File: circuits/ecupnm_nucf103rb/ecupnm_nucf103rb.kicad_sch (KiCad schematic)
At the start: 45 parts, among them J1 Conn_01x02_Pin, J2 Conn_01x02_Pin, J3 Conn_01x02_Pin, J4 Conn_01x03_Pin, J5 USB_B_Mini, U1 NUCLEO-64, U3 AMS1117-5.0

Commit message: Nucleo 64
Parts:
- C4: footprint (none) -> Capacitor_SMD:C_1206_3216Metric_Pad1.33x1.80mm_HandSolder
- C? (x4): footprint Capacitor_SMD:C_0805_2012Metric_Pad1.18x1.45mm_HandSolder -> Capacitor_SMD:C_1206_3216Metric_Pad1.33x1.80mm_HandSolder
- D3: footprint (none) -> LED_SMD:LED_1206_3216Metric_Pad1.42x1.75mm_HandSolder
- D?: footprint LED_SMD:LED_0805_2012Metric_Pad1.15x1.40mm_HandSolder -> LED_SMD:LED_1206_3216Metric_Pad1.42x1.75mm_HandSolder
- J1, J2, J3: footprint (none) -> Connector_PinSocket_2.54mm:PinSocket_1x02_P2.54mm_Vertical
- J4: footprint (none) -> Connector_PinSocket_2.54mm:PinSocket_1x03_P2.54mm_Vertical
- J5: footprint (none) -> Connector_USB:USB_Mini-B_Wuerth_65100516121_Horizontal
- JT1: footprint (none) -> TerminalBlock:TerminalBlock_Altech_AK300-3_P5.00mm
- JT2, JT3: footprint (none) -> TerminalBlock:TerminalBlock_Altech_AK300-2_P5.00mm
- R8, R9: footprint (none) -> Resistor_SMD:R_1206_3216Metric_Pad1.30x1.75mm_HandSolder
- R? (x13): footprint Resistor_SMD:R_0805_2012Metric_Pad1.20x1.40mm_HandSolder -> Resistor_SMD:R_1206_3216Metric_Pad1.30x1.75mm_HandSolder
- U1: footprint MODULE -> user:Nucleo-64
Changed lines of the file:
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@@
       (effects (font (size 1.27 1.27)))
     )
-    (property "Footprint" "" (at 139.7 51.1048 0)
+    (property "Footprint" "Capacitor_SMD:C_1206_3216Metric_Pad1.33x1.80mm_HandSolder" (at 139.7 51.1048 0)
       (effects (font (size 1.27 1.27)) hide)
     )
@@
       (effects (font (size 1.27 1.27)) hide)
     )
-    (property "Footprint" "" (at 114.3 119.38 0)
+    (property "Footprint" "Connector_PinSocket_2.54mm:PinSocket_1x02_P2.54mm_Vertical" (at 114.3 119.38 0)
       (effects (font (size 1.27 1.27)) hide)
     )
@@
       (effects (font (size 1.27 1.27)) (justify left))
     )
-    (property "Footprint" "Resistor_SMD:R_0805_2012Metric_Pad1.20x1.40mm_HandSolder" (at 94.742 104.14 90)
+    (property "Footprint" "Resistor_SMD:R_1206_3216Metric_Pad1.30x1.75mm_HandSolder" (at 94.742 104.14 90)
       (effects (font (size 1.27 1.27)) hide)
     )
@@
       (effects (font (size 1.27 1.27)) (justify left))
     )
-    (property "Footprint" "Resistor_SMD:R_0805_2012Metric_Pad1.20x1.40mm_HandSolder" (at 122.682 104.14 90)
+    (property "Footprint" "Resistor_SMD:R_1206_3216Metric_Pad1.30x1.75mm_HandSolder" (at 122.682 104.14 90)
       (effects (font (size 1.27 1.27)) hide)
     )
@@
       (effects (font (size 1.27 1.27)) (justify left))
     )
-    (property "Footprint" "Capacitor_SMD:C_0805_2012Metric_Pad1.18x1.45mm_HandSolder" (at 105.1052 175.26 0)
+    (property "Footprint" "Capacitor_SMD:C_1206_3216Metric_Pad1.33x1.80mm_HandSolder" (at 105.1052 175.26 0)
       (effects (font (size 1.27 1.27)) hide)
     )
@@
       (effects (font (size 1.27 1.27)) hide)
     )
-    (property "Footprint" "" (at 30.48 166.37 0)
+    (property "Footprint" "TerminalBlock:TerminalBlock_Altech_AK300-3_P5.00mm" (at 30.48 166.37 0)
       (effects (font (size 1.27 1.27)) hide)
     )
@@
       (effects (font (size 1.27 1.27)) (justify right))
     )
-    (property "Footprint" "LED_SMD:LED_0805_2012Metric_Pad1.15x1.40mm_HandSolder" (at 88.9 114.3 0)
+    (property "Footprint" "LED_SMD:LED_1206_3216Metric_Pad1.42x1.75mm_HandSolder" (at 88.9 114.3 0)
       (effects (font (size 1.27 1.27)) hide)
     )
@@
       (effects (font (size 1.27 1.27)))
     )
-    (property "Footprint" "Resistor_SMD:R_0805_2012Metric_Pad1.20x1.40mm_HandSolder" (at 166.37 47.498 90)
+    (property "Footprint" "Resistor_SMD:R_1206_3216Metric_Pad1.30x1.75mm_HandSolder" (at 166.37 47.498 90)
       (effects (font (size 1.27 1.27)) hide)
     )
@@
       (effects (font (size 1.27 1.27)) hide)
     )
-    (property "Footprint" "" (at 86.36 162.56 0)
+    (property "Footprint" "TerminalBlock:TerminalBlock_Altech_AK300-2_P5.00mm" (at 86.36 162.56 0)
       (effects (font (size 1.27 1.27)) hide)
     )
@@
       (effects (font (size 1.27 1.27)))
     )
-    (property "Footprint" "Resistor_SMD:R_0805_2012Metric_Pad1.20x1.40mm_HandSolder" (at 223.52 47.498 90)
+    (property "Footprint" "Resistor_SMD:R_1206_3216Metric_Pad1.30x1.75mm_HandSolder" (at 223.52 47.498 90)
       (effects (font (size 1.27 1.27)) hide)
     )
@@
       (effects (font (size 1.27 1.27)) (justify left))
     )
-    (property "Footprint" "Resistor_SMD:R_0805_2012Metric_Pad1.20x1.40mm_HandSolder" (at 74.422 120.65 90)
+    (property "Footprint" "Resistor_SMD:R_1206_3216Metric_Pad1.30x1.75mm_HandSolder" (at 74.422 120.65 90)
       (effects (font (size 1.27 1.27)) hide)
     )
@@
       (effects (font (size 1.27 1.27)))
     )
-    (property "Footprint" "MODULE" (at 113.03 22.86 0)
+    (property "Footprint" "user:Nucleo-64" (at 113.03 22.86 0)
       (effects (font (size 1.27 1.27)) hide)
     )
@@
       (effects (font (size 1.27 1.27)) hide)
     )
-    (property "Footprint" "" (at 114.3 129.54 0)
+    (property "Footprint" "Connector_PinSocket_2.54mm:PinSocket_1x03_P2.54mm_Vertical" (at 114.3 129.54 0)
       (effects (font (size 1.27 1.27)) hide)
     )
@@
       (effects (font (size 1.27 1.27)) (justify left))
     )
-    (property "Footprint" "Capacitor_SMD:C_0805_2012Metric_Pad1.18x1.45mm_HandSolder" (at 48.5648 168.91 0)
+    (property "Footprint" "Capacitor_SMD:C_1206_3216Metric_Pad1.33x1.80mm_HandSolder" (at 48.5648 168.91 0)
       (effects (font (size 1.27 1.27)) hide)
     )
@@
       (effects (font (size 1.27 1.27)) (justify left))
     )
-    (property "Footprint" "Resistor_SMD:R_0805_2012Metric_Pad1.20x1.40mm_HandSolder" (at 245.872 41.91 90)
+    (property "Footprint" "Resistor_SMD:R_1206_3216Metric_Pad1.30x1.75mm_HandSolder" (at 245.872 41.91 90)
       (effects (font (size 1.27 1.27)) hide)
     )
@@
       (effects (font (size 1.27 1.27)))
     )
-    (property "Footprint" "" (at 171.45 97.79 0)
+    (property "Footprint" "Connector_USB:USB_Mini-B_Wuerth_65100516121_Horizontal" (at 171.45 97.79 0)
       (effects (font (size 1.27 1.27)) hide)
     )
@@
       (effects (font (size 1.27 1.27)) hide)
     )
-    (property "Footprint" "" (at 31.75 180.34 0)
+    (property "Footprint" "Connector_PinSocket_2.54mm:PinSocket_1x02_P2.54mm_Vertical" (at 31.75 180.34 0)
       (effects (font (size 1.27 1.27)) hide)
     )
@@
       (effects (font (size 1.27 1.27)))
     )
-    (property "Footprint" "Resistor_SMD:R_0805_2012Metric_Pad1.20x1.40mm_HandSolder" (at 45.72 168.148 90)
+    (property "Footprint" "Resistor_SMD:R_1206_3216Metric_Pad1.30x1.75mm_HandSolder" (at 45.72 168.148 90)
       (effects (font (size 1.27 1.27)) hide)
     )
@@
       (effects (font (size 1.27 1.27)) (justify left))
     )
-    (property "Footprint" "Capacitor_SMD:C_0805_2012Metric_Pad1.18x1.45mm_HandSolder" (at 133.6548 167.64 0)
+    (property "Footprint" "Capacitor_SMD:C_1206_3216Metric_Pad1.33x1.80mm_HandSolder" (at 133.6548 167.64 0)
       (effects (font (size 1.27 1.27)) hide)
     )
@@
       (effects (font (size 1.27 1.27)))
     )
-    (property "Footprint" "" (at 135.89 58.928 90)
+    (property "Footprint" "Resistor_SMD:R_1206_3216Metric_Pad1.30x1.75mm_HandSolder" (at 135.89 58.928 90)
       (effects (font (size 1.27 1.27)) hide)
     )
@@
       (effects (font (size 1.27 1.27)) (justify left))
     )
-    (property "Footprint" "Resistor_SMD:R_0805_2012Metric_Pad1.20x1.40mm_HandSolder" (at 197.612 36.83 90)
+    (property "Footprint" "Resistor_SMD:R_1206_3216Metric_Pad1.30x1.75mm_HandSolder" (at 197.612 36.83 90)
       (effects (font (size 1.27 1.27)) hide)
     )
@@
       (effects (font (size 1.27 1.27)) (justify right))
     )
-    (property "Footprint" "Resistor_SMD:R_0805_2012Metric_Pad1.20x1.40mm_HandSolder" (at 57.658 172.72 90)
+    (property "Footprint" "Resistor_SMD:R_1206_3216Metric_Pad1.30x1.75mm_HandSolder" (at 57.658 172.72 90)
       (effects (font (size 1.27 1.27)) hide)
     )
@@
       (effects (font (size 1.27 1.27)) hide)
     )
-    (property "Footprint" "" (at 220.98 26.67 0)
+    (property "Footprint" "TerminalBlock:TerminalBlock_Altech_AK300-2_P5.00mm" (at 220.98 26.67 0)
       (effects (font (size 1.27 1.27)) hide)
     )
@@
       (effects (font (size 1.27 1.27)) (justify left))
     )
-    (property "Footprint" "Resistor_SMD:R_0805_2012Metric_Pad1.20x1.40mm_HandSolder" (at 188.722 41.91 90)
+    (property "Footprint" "Resistor_SMD:R_1206_3216Metric_Pad1.30x1.75mm_HandSolder" (at 188.722 41.91 90)
       (effects (font (size 1.27 1.27)) hide)
     )
@@
       (effects (font (size 1.27 1.27)) (justify left))
     )
-    (property "Footprint" "" (at 139.192 104.14 90)
+    (property "Footprint" "Resistor_SMD:R_1206_3216Metric_Pad1.30x1.75mm_HandSolder" (at 139.192 104.14 90)
       (effects (font (size 1.27 1.27)) hide)
     )
@@
       (effects (font (size 1.27 1.27)) (justify right))
     )
-    (property "Footprint" "" (at 140.97 111.76 0)
+    (property "Footprint" "LED_SMD:LED_1206_3216Metric_Pad1.42x1.75mm_HandSolder" (at 140.97 111.76 0)
       (effects (font (size 1.27 1.27)) hide)
     )
@@
       (effects (font (size 1.27 1.27)) (justify left))
     )
-    (property "Footprint" "Resistor_SMD:R_0805_2012Metric_Pad1.20x1.40mm_HandSolder" (at 254.762 36.83 90)
+    (property "Footprint" "Resistor_SMD:R_1206_3216Metric_Pad1.30x1.75mm_HandSolder" (at 254.762 36.83 90)
       (effects (font (size 1.27 1.27)) hide)
     )
@@
       (effects (font (size 1.27 1.27)))
     )
-    (property "Footprint" "MODULE" (at 52.07 22.86 0)
+    (property "Footprint" "user:Nucleo-64" (at 52.07 22.86 0)
       (effects (font (size 1.27 1.27)) hide)
     )
@@
       (effects (font (size 1.27 1.27)) (justify left))
     )
-    (property "Footprint" "Resistor_SMD:R_0805_2012Metric_Pad1.20x1.40mm_HandSolder" (at 87.122 104.14 90)
+    (property "Footprint" "Resistor_SMD:R_1206_3216Metric_Pad1.30x1.75mm_HandSolder" (at 87.122 104.14 90)
       (effects (font (size 1.27 1.27)) hide)
     )
@@
       (effects (font (size 1.27 1.27)) (justify left))
     )
-    (property "Footprint" "Resistor_SMD:R_0805_2012Metric_Pad1.20x1.40mm_HandSolder" (at 79.502 134.62 90)
+    (property "Footprint" "Resistor_SMD:R_1206_3216Metric_Pad1.30x1.75mm_HandSolder" (at 79.502 134.62 90)
       (effects (font (size 1.27 1.27)) hide)
     )
@@
       (effects (font (size 1.27 1.27)) hide)
     )
-    (property "Footprint" "" (at 64.77 96.52 0)
+    (property "Footprint" "Connector_PinSocket_2.54mm:PinSocket_1x02_P2.54mm_Vertical" (at 64.77 96.52 0)
       (effects (font (size 1.27 1.27)) hide)
     )
@@
       (effects (font (size 1.27 1.27)) (justify left))
     )
-    (property "Footprint" "Capacitor_SMD:C_0805_2012Metric_Pad1.18x1.45mm_HandSolder" (at 75.2348 130.81 0)
-      (effects (font (size 1.27 1.27)) hide)
-    )
+    (property "Footprint" "Capacitor_SMD:C_1206_3216Metric_Pad1.33x1.80mm_HandSolder" (at 75.2348 130.81 0)
+      (effects (font (size 1.27 1.27)) hide)
+    )

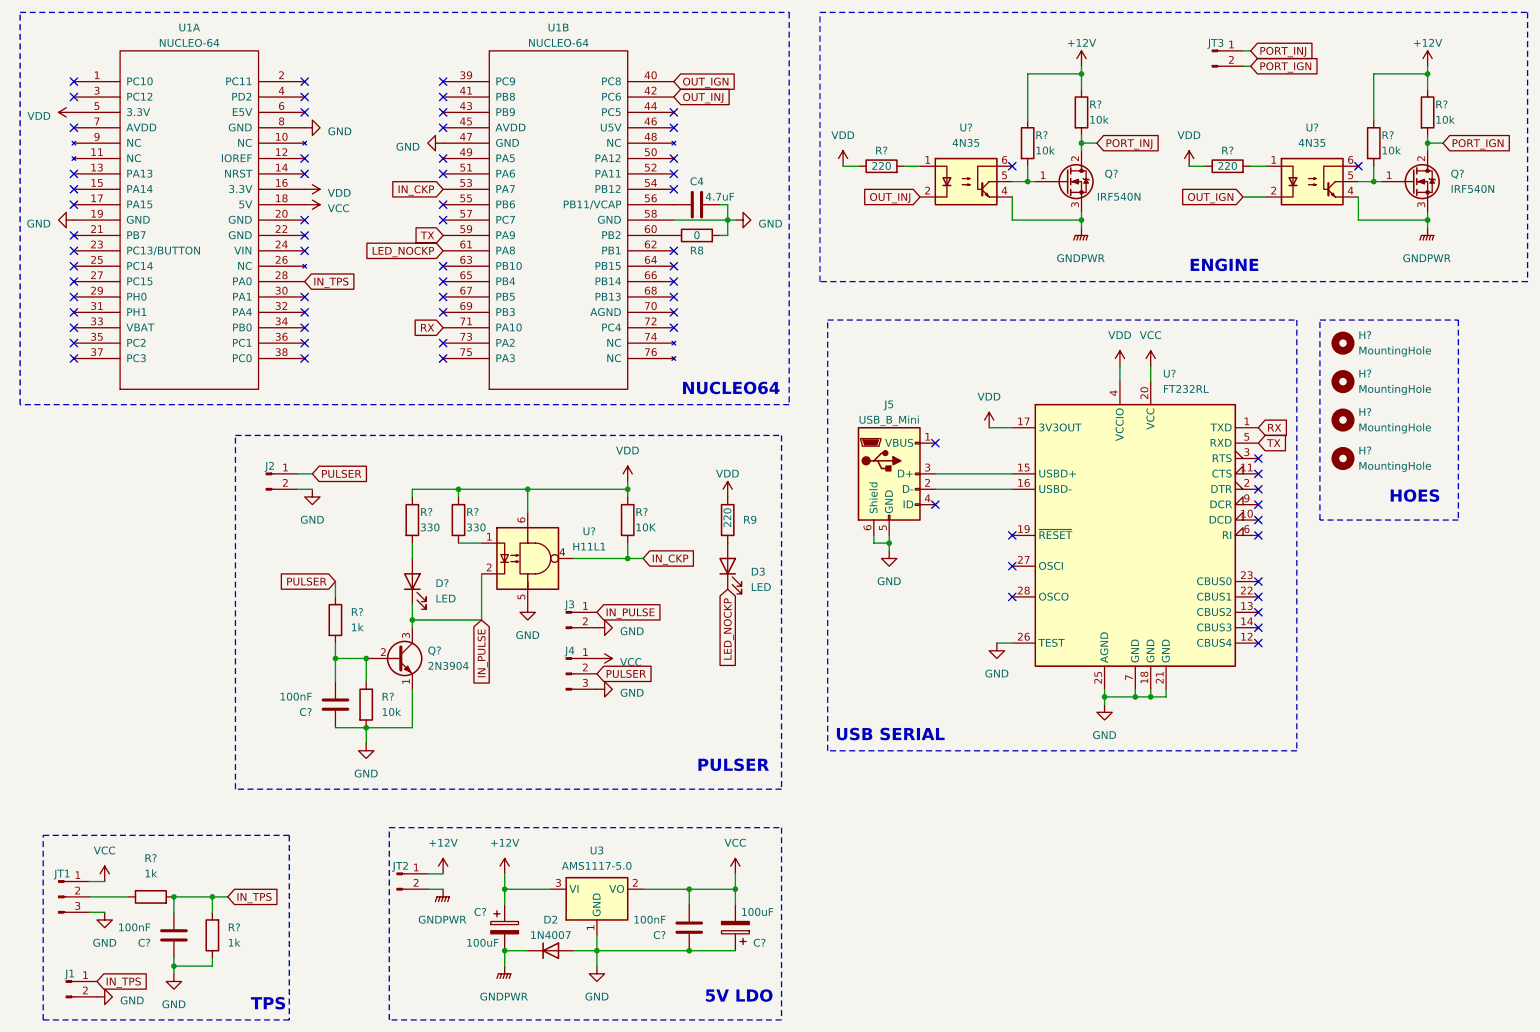
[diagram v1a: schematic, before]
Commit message: ECU Nucleo Based
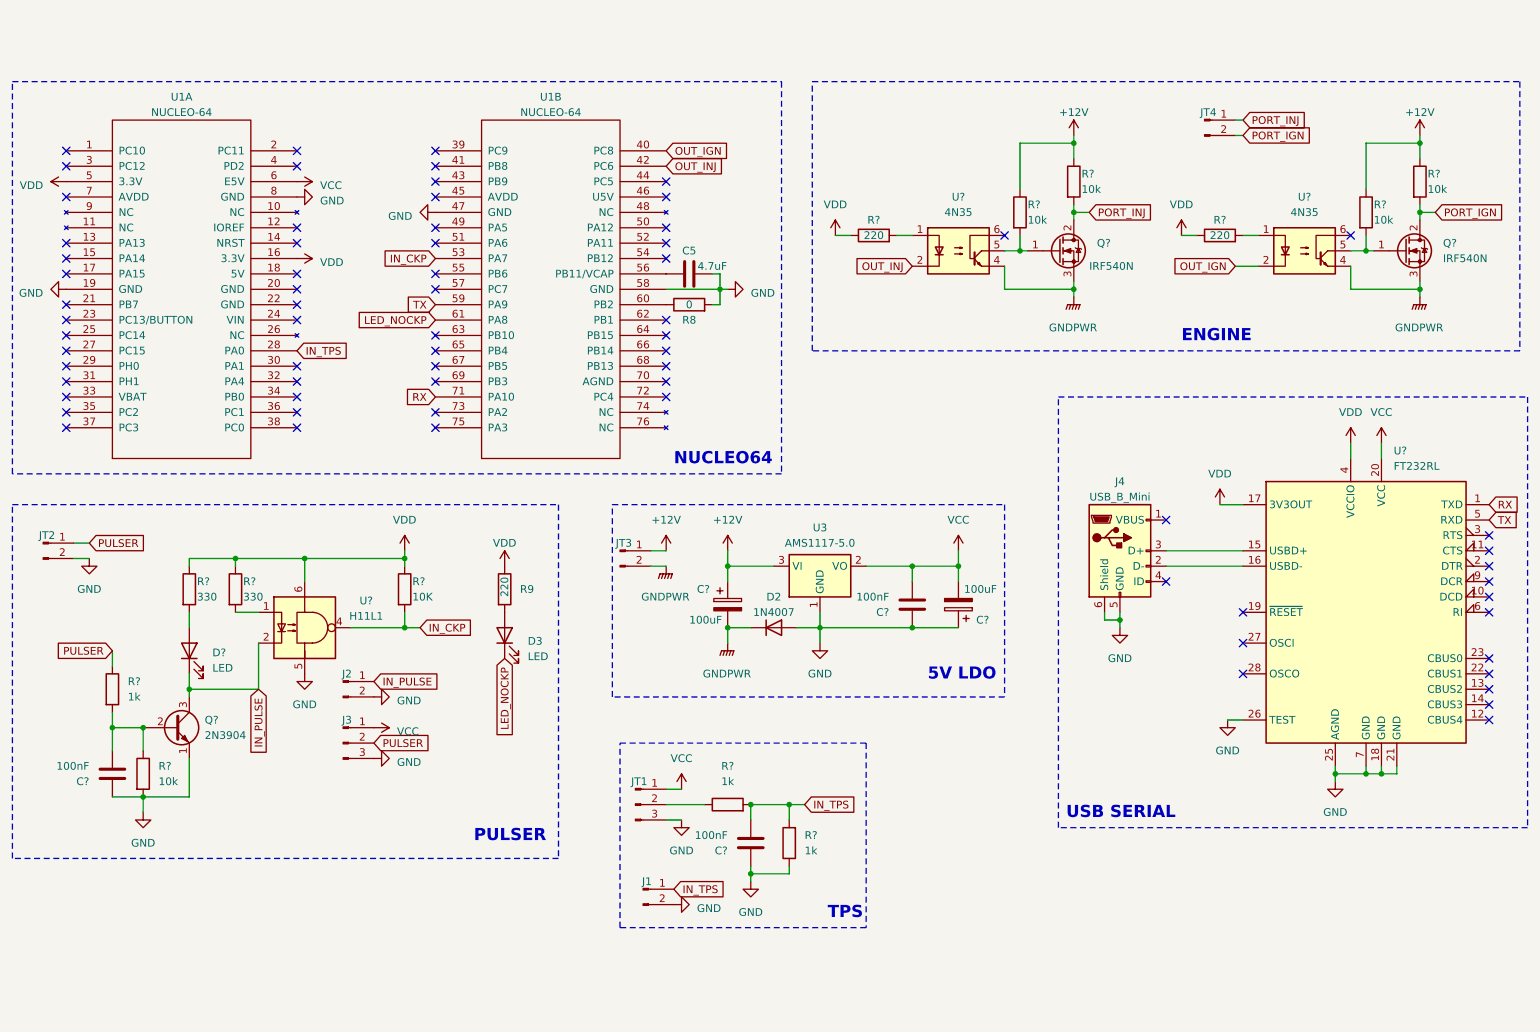
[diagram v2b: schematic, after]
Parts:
- removed H? (x4): MountingHole, MountingHole:MountingHole_2.5mm_Pad, symbol Mechanical:MountingHole
- C?: footprint Capacitor_SMD:C_1206_3216Metric_Pad1.33x1.80mm_HandSolder -> Capacitor_SMD:CP_Elec_4x5.4
- J1: footprint Connector_PinSocket_2.54mm:PinSocket_1x02_P2.54mm_Vertical -> Connector_PinHeader_2.54mm:PinHeader_1x02_P2.54mm_Vertical
- J2: renamed from J3; footprint Connector_PinSocket_2.54mm:PinSocket_1x02_P2.54mm_Vertical -> Connector_PinHeader_2.54mm:PinHeader_1x02_P2.54mm_Vertical
- J3: renamed from J4; footprint Connector_PinSocket_2.54mm:PinSocket_1x03_P2.54mm_Vertical -> Connector_PinHeader_2.54mm:PinHeader_1x03_P2.54mm_Vertical
- JT2: renamed from J2; footprint Connector_PinSocket_2.54mm:PinSocket_1x02_P2.54mm_Vertical -> TerminalBlock:TerminalBlock_Altech_AK300-2_P5.00mm
- Q? (x2): footprint Package_TO_SOT_THT:TO-220-3_Horizontal_TabUp -> Package_TO_SOT_THT:TO-220-3_Horizontal_TabDown
- renumbered C4 to C5, J5 to J4, JT2 to JT3, JT3 to JT4
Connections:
- net VCC: now also U1.6 (E5V); no longer U1.18 (5V)
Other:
- note removed: "HOES"
- moved on the sheet: C5, C?, D2, D3, D?, J1, J2, J3, J4, JT1, JT2, JT3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
